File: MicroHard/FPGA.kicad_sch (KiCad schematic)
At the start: 1 part

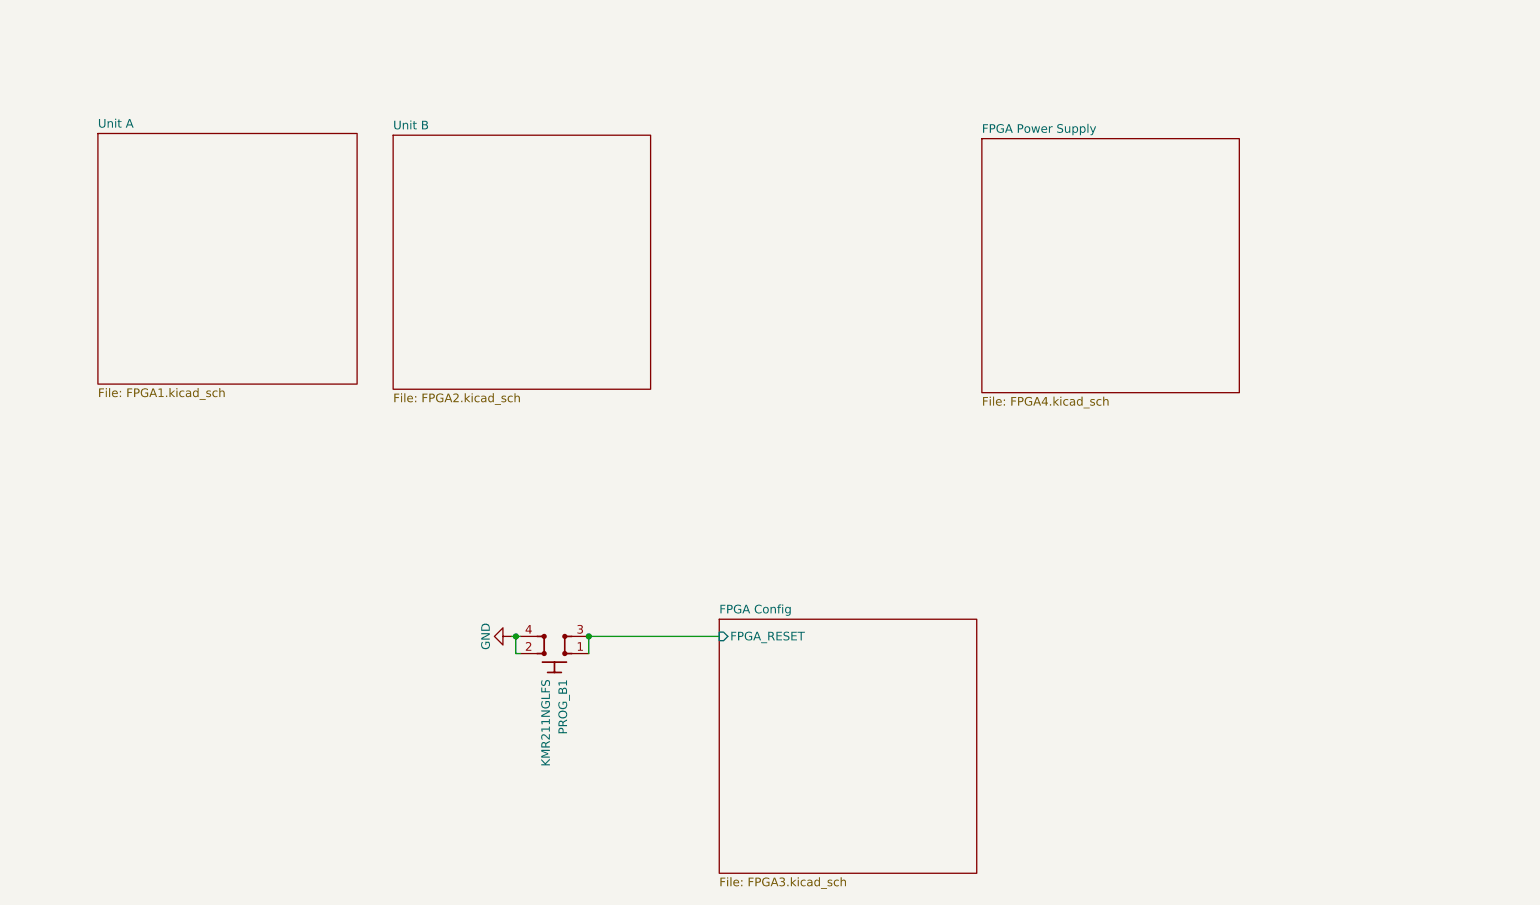
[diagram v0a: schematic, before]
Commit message: feat: finished Flash mem and FPGA Config
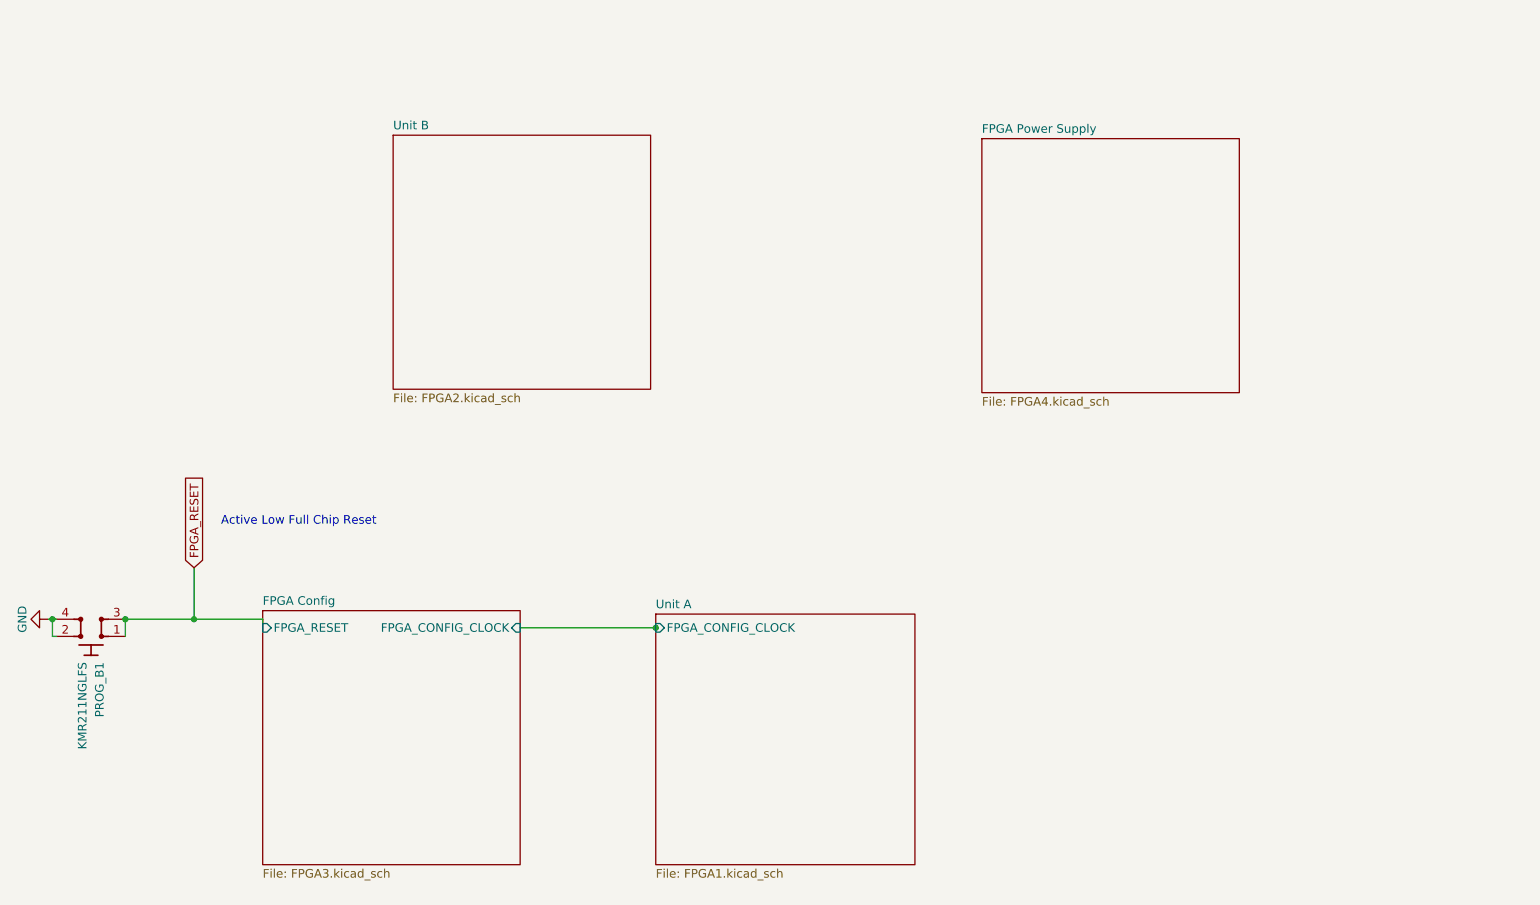
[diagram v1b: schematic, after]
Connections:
- net FPGA Config/FPGA_RESET renamed FPGA_RESET
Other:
- sheet FPGA Config ports: added FPGA_CONFIG_CLOCK; removed none
- sheet Unit A ports: added FPGA_CONFIG_CLOCK; removed none
- note added: "Active Low Full Chip Reset"
- moved on the sheet: PROG_B1
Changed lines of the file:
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@@
 	(paper "A4")
 	(junction
-		(at 94.615 115.57)
+		(at 46.99 113.03)
 		(diameter 0)
 		(color 0 0 0 0)
 	)
 	(junction
-		(at 105.41 115.57)
+		(at 26.035 113.03)
 		(diameter 0)
 		(color 0 0 0 0)
 	)
-	(wire
-		(pts
-			(xy 94.615 118.11) (xy 95.25 118.11)
-		)
-		(stroke
-			(width 0)
-			(type default)
-		)
-	)
-	(wire
-		(pts
-			(xy 94.615 115.57) (xy 95.25 115.57)
-		)
-		(stroke
-			(width 0)
-			(type default)
-		)
-	)
-	(wire
-		(pts
-			(xy 105.41 115.57) (xy 124.714 115.57)
-		)
-		(stroke
-			(width 0)
-			(type default)
-		)
-	)
-	(wire
-		(pts
-			(xy 105.41 115.57) (xy 105.41 118.11)
-		)
-		(stroke
-			(width 0)
-			(type default)
-		)
-	)
-	(wire
-		(pts
-			(xy 94.615 118.11) (xy 94.615 115.57)
-		)
-		(stroke
-			(width 0)
-			(type default)
-		)
-	)
-	(wire
-		(pts
-			(xy 94.615 115.57) (xy 93.98 115.57)
-		)
-		(stroke
-			(width 0)
-			(type default)
+	(junction
+		(at 36.83 113.03)
+		(diameter 0)
+		(color 0 0 0 0)
+	)
+	(junction
+		(at 115.316 114.3)
+		(diameter 0)
+		(color 0 0 0 0)
+	)
+	(wire
+		(pts
+			(xy 57.15 113.03) (xy 46.99 113.03)
+		)
+		(stroke
+			(width 0)
+			(type default)
+		)
+	)
+	(wire
+		(pts
+			(xy 26.035 115.57) (xy 26.67 115.57)
+		)
+		(stroke
+			(width 0)
+			(type default)
+		)
+	)
+	(wire
+		(pts
+			(xy 26.035 113.03) (xy 26.67 113.03)
+		)
+		(stroke
+			(width 0)
+			(type default)
+		)
+	)
+	(wire
+		(pts
+			(xy 36.83 113.03) (xy 46.99 113.03)
+		)
+		(stroke
+			(width 0)
+			(type default)
+		)
+	)
+	(wire
+		(pts
+			(xy 115.316 114.3) (xy 115.57 114.3)
+		)
+		(stroke
+			(width 0)
+			(type default)
+		)
+	)
+	(wire
+		(pts
+			(xy 46.99 105.41) (xy 46.99 113.03)
+		)
+		(stroke
+			(width 0)
+			(type default)
+		)
+	)
+	(wire
+		(pts
+			(xy 36.83 113.03) (xy 36.83 115.57)
+		)
+		(stroke
+			(width 0)
+			(type default)
+		)
+	)
+	(wire
+		(pts
+			(xy 95.25 114.3) (xy 115.316 114.3)
+		)
+		(stroke
+			(width 0)
+			(type default)
+		)
+	)
+	(wire
+		(pts
+			(xy 57.15 113.03) (xy 57.15 114.3)
+		)
+		(stroke
+			(width 0)
+			(type default)
+		)
+	)
+	(wire
+		(pts
+			(xy 26.035 115.57) (xy 26.035 113.03)
+		)
+		(stroke
+			(width 0)
+			(type default)
+		)
+	)
+	(wire
+		(pts
+			(xy 26.035 113.03) (xy 25.4 113.03)
+		)
+		(stroke
+			(width 0)
+			(type default)
+		)
+	)
+	(text "Active Low Full Chip Reset"
+		(exclude_from_sim no)
+		(at 62.484 98.552 0)
+		(effects
+			(font
+				(size 1.27 1.27)
+			)
+		)
+	)
+	(global_label "FPGA_RESET"
+		(shape input)
+		(at 46.99 105.41 90)
+		(fields_autoplaced yes)
+		(effects
+			(font
+				(size 1.27 1.27)
+			)
+			(justify left)
+		)
+		(property "Intersheetrefs" "${INTERSHEET_REFS}"
+			(at 46.99 90.9949 90)
+			(effects
+				(font
+					(size 1.27 1.27)
+				)
+				(justify left)
+				(hide yes)
+			)
 		)
 	)
 	(symbol
 		(lib_id "antmicroPushbuttonSwitches:SW_SPST_KMR211NGLFS")
-		(at 105.41 118.11 180)
+		(at 36.83 115.57 180)
 		(unit 1)
 		(exclude_from_sim no)
@@
 		(fields_autoplaced yes)
 		(property "Reference" "PROG_B1"
-			(at 101.6001 121.92 90)
+			(at 33.0201 119.38 90)
 			(effects
 				(font
@@
 		)
 		(property "Value" "SW_SPST_KMR211NGLFS"
-			(at 99.0601 121.92 90)
+			(at 30.4801 119.38 90)
 			(effects
 				(font
@@
 		)
 		(property "Footprint" "antmicro-footprints:SW_SPST_4.2x2.8"
-			(at 80.01 110.49 0)
+			(at 11.43 107.95 0)
 			(effects
 				(font
@@
 		)
 		(property "Datasheet" "http://www.farnell.com/datasheets/2631211.pdf"
-			(at 80.01 107.95 0)
+			(at 11.43 105.41 0)
 			(effects
 				(font
@@
 		)
 		(property "Description" ""
-			(at 105.41 118.11 0)
+			(at 36.83 115.57 0)
 			(effects
 				(font
@@
 		)
 		(property "MPN" "KMR211NGLFS"
-			(at 99.0601 121.92 90)
+			(at 30.4801 119.38 90)
 			(effects
 				(font
@@
 		)
 		(property "Manufacturer" "C&K"
-			(at 80.01 102.87 0)
+			(at 11.43 100.33 0)
 			(effects
 				(font
@@
 		)
 		(property "Author" "Antmicro"
-			(at 80.01 100.33 0)
+			(at 11.43 97.79 0)
 			(effects
 				(font
@@
 		)
 		(property "License" "Apache-2.0"
-			(at 80.01 97.79 0)
+			(at 11.43 95.25 0)
 			(effects
 				(font
@@
 	(symbol
 		(lib_id "antmicropower:GND")
-		(at 93.98 115.57 270)
+		(at 25.4 113.03 270)
 		(unit 1)
 		(exclude_from_sim no)
@@
 		(dnp no)
 		(property "Reference" "#PWR018"
-			(at 87.63 115.57 0)
+			(at 19.05 113.03 0)
 			(effects
 				(font
@@
 		)
 		(property "Value" "GND"
-			(at 90.17 115.57 0)
+			(at 21.59 113.03 0)
 			(effects
 				(font
@@
 		)
 		(property "Footprint" ""
-			(at 93.98 115.57 0)
+			(at 25.4 113.03 0)
 			(effects
 				(font
@@
 		)
 		(property "Datasheet" ""
-			(at 93.98 115.57 0)
+			(at 25.4 113.03 0)
 			(effects
 				(font
@@
 		)
 		(property "Description" ""
-			(at 93.98 115.57 0)
+			(at 25.4 113.03 0)
 			(effects
 				(font
@@
 		)
 		(property "Author" "Antmicro"
-			(at 86.36 124.46 0)
+			(at 17.78 121.92 0)
 			(effects
 				(font
@@
 		)
 		(property "License" "Apache-2.0"
-			(at 83.82 124.46 0)
+			(at 15.24 121.92 0)
 			(effects
 				(font
@@
 	)
 	(sheet
-		(at 32.766 41.148)
+		(at 115.316 112.268)
 		(size 38.354 37.084)
 		(fields_autoplaced yes)
@@
 		)
 		(property "Sheetname" "Unit A"
-			(at 32.766 40.4364 0)
+			(at 115.316 111.5564 0)
 			(effects
 				(font
@@
 		)
 		(property "Sheetfile" "FPGA1.kicad_sch"
-			(at 32.766 78.8166 0)
+			(at 115.316 149.9366 0)
 			(effects
 				(font
@@
 				)
 				(justify left top)
+			)
+		)
+		(pin "FPGA_CONFIG_CLOCK" input
+			(at 115.316 114.3 180)
+			(effects
+				(font
+					(size 1.27 1.27)
+				)
+				(justify left)
 			)
 		)
@@
 	)
 	(sheet
-		(at 124.714 113.03)
+		(at 57.15 111.76)
 		(size 38.1 37.592)
 		(fields_autoplaced yes)
@@
 		)
 		(property "Sheetname" "FPGA Config"
-			(at 124.714 112.3184 0)
+			(at 57.15 111.0484 0)
 			(effects
 				(font
@@
 		)
 		(property "Sheetfile" "FPGA3.kicad_sch"
-			(at 124.714 151.2066 0)
+			(at 57.15 149.9366 0)
 			(effects
 				(font
@@
 		)
 		(pin "FPGA_RESET" input
-			(at 124.714 115.57 180)
-			(effects
-				(font
-					(size 1.27 1.27)
-				)
-				(justify left)
-			)
-		)
+			(at 57.15 114.3 180)
+			(effects
+				(font
+					(size 1.27 1.27)
+				)
+				(justify left)
+			)
+		)
+		(pin "FPGA_CONFIG_CLOCK" input
+			(at 95.25 114.3 0)
+			(effects
+				(font
+					(size 1.27 1.27)
+				)
+				(justify right)
+			)
+		)

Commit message: feat: finished config
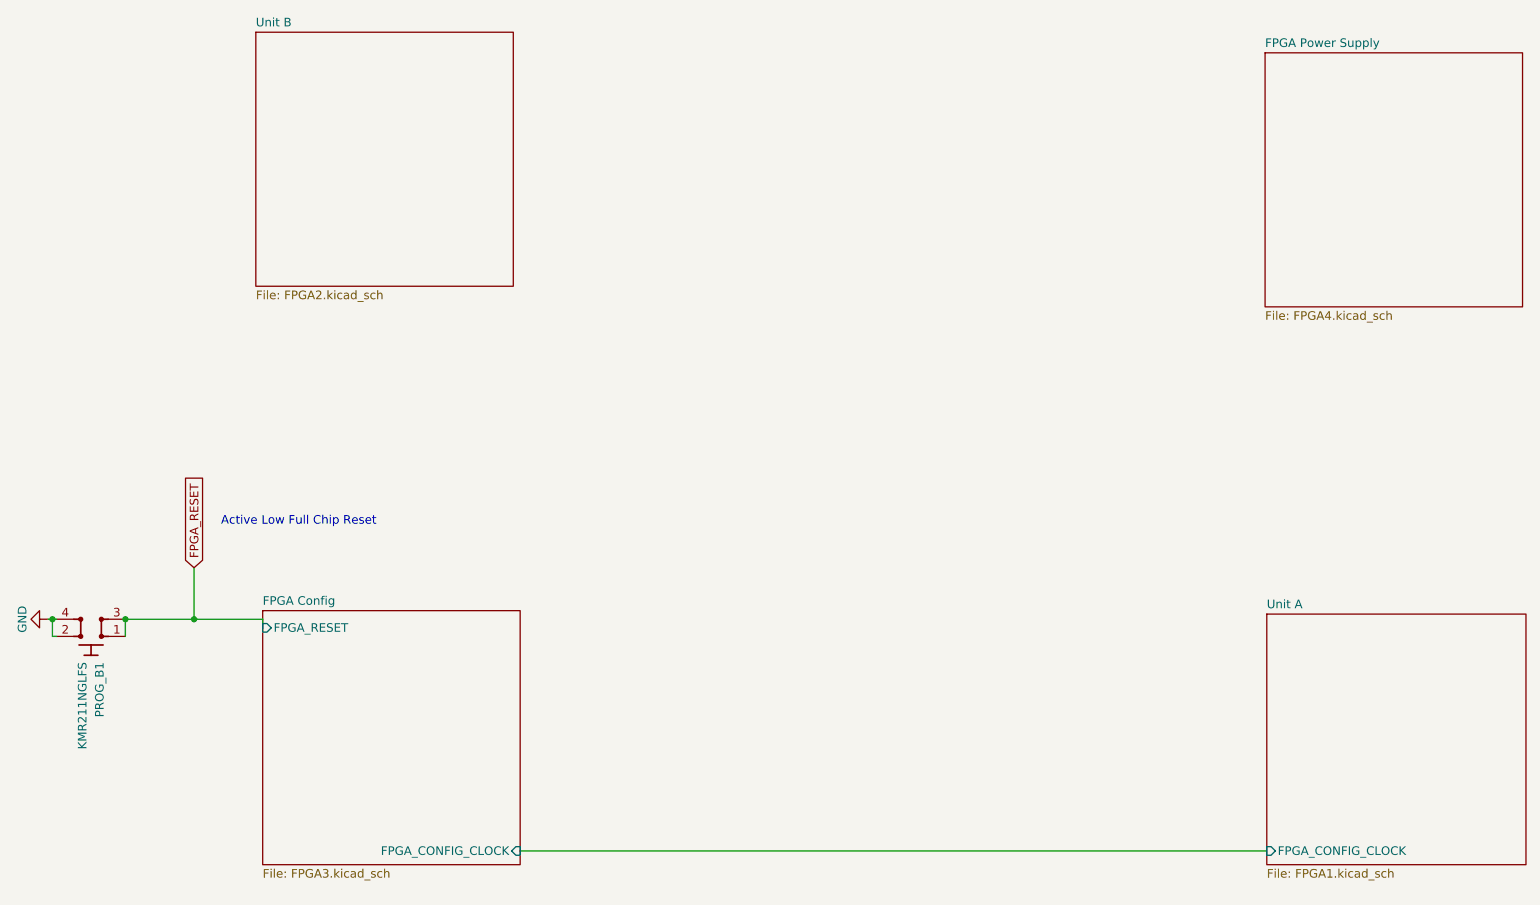
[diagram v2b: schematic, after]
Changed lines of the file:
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@@
 		(color 0 0 0 0)
 	)
-	(junction
-		(at 115.316 114.3)
-		(diameter 0)
-		(color 0 0 0 0)
-	)
 	(wire
 		(pts
@@
 	(wire
 		(pts
-			(xy 115.316 114.3) (xy 115.57 114.3)
+			(xy 95.25 147.32) (xy 205.74 147.32)
 		)
 		(stroke
@@
 		(pts
 			(xy 36.83 113.03) (xy 36.83 115.57)
-		)
-		(stroke
-			(width 0)
-			(type default)
-		)
-	)
-	(wire
-		(pts
-			(xy 95.25 114.3) (xy 115.316 114.3)
 		)
 		(stroke
@@
 	)
 	(sheet
-		(at 115.316 112.268)
+		(at 205.74 112.268)
 		(size 38.354 37.084)
 		(fields_autoplaced yes)
@@
 		)
 		(property "Sheetname" "Unit A"
-			(at 115.316 111.5564 0)
+			(at 205.74 111.5564 0)
 			(effects
 				(font
@@
 		)
 		(property "Sheetfile" "FPGA1.kicad_sch"
-			(at 115.316 149.9366 0)
+			(at 205.74 149.9366 0)
 			(effects
 				(font
@@
 		)
 		(pin "FPGA_CONFIG_CLOCK" input
-			(at 115.316 114.3 180)
+			(at 205.74 147.32 180)
 			(effects
 				(font
@@
 	)
 	(sheet
-		(at 76.454 41.402)
+		(at 56.134 26.162)
 		(size 38.1 37.592)
 		(fields_autoplaced yes)
@@
 		)
 		(property "Sheetname" "Unit B"
-			(at 76.454 40.6904 0)
+			(at 56.134 25.4504 0)
 			(effects
 				(font
@@
 		)
 		(property "Sheetfile" "FPGA2.kicad_sch"
-			(at 76.454 79.5786 0)
+			(at 56.134 64.3386 0)
 			(effects
 				(font
@@
 		)
 		(pin "FPGA_CONFIG_CLOCK" input
-			(at 95.25 114.3 0)
+			(at 95.25 147.32 0)
 			(effects
 				(font
@@
 	)
 	(sheet
-		(at 163.576 41.91)
+		(at 205.486 29.21)
 		(size 38.1 37.592)
 		(fields_autoplaced yes)
@@
 		)
 		(property "Sheetname" "FPGA Power Supply"
-			(at 163.576 41.1984 0)
+			(at 205.486 28.4984 0)
 			(effects
 				(font
@@
 		)
 		(property "Sheetfile" "FPGA4.kicad_sch"
-			(at 163.576 80.0866 0)
-			(effects
-				(font
+			(at 205.486 67.3866 0)
+			(effects
+				(font
